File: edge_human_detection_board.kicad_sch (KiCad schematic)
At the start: 1 part

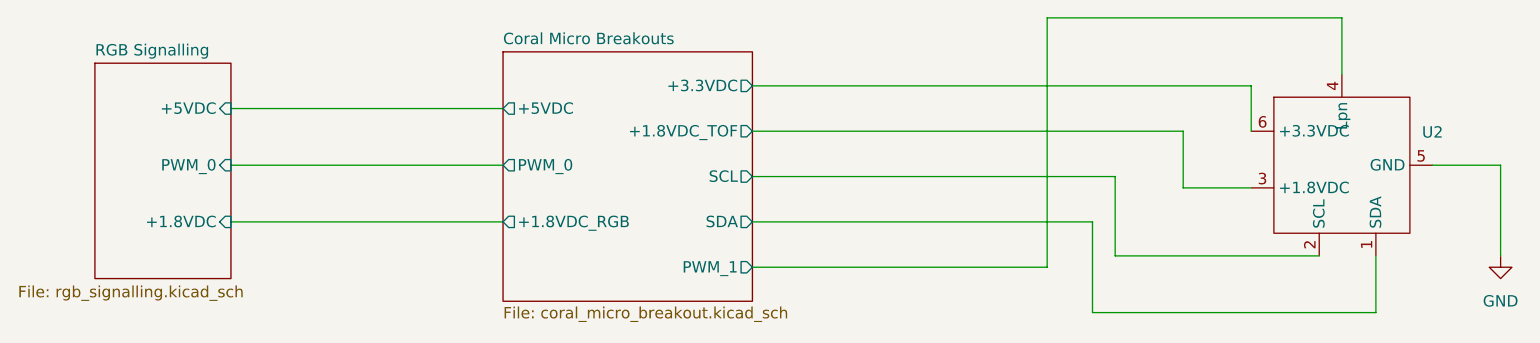
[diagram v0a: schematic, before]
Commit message: latest updates, up to v2
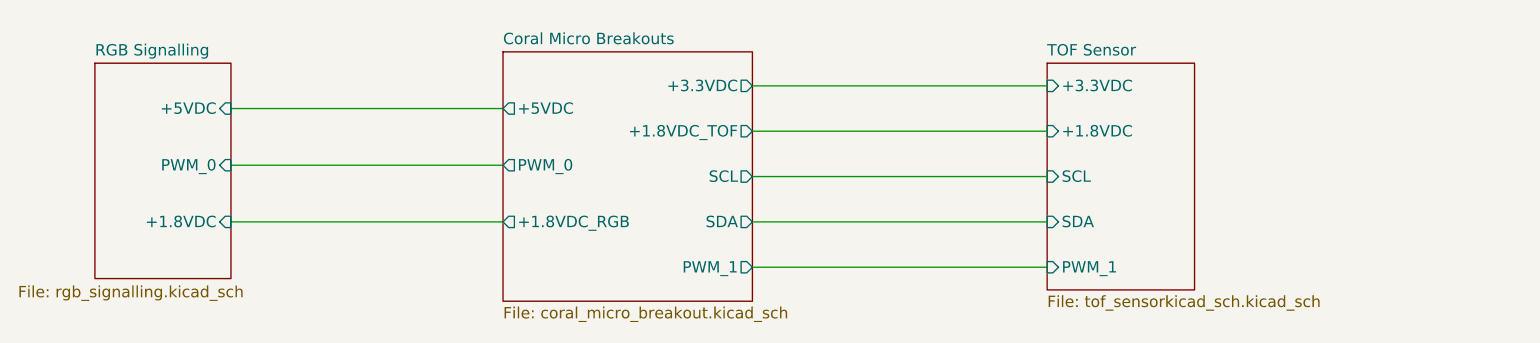
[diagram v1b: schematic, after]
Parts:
- removed U2: ~, 00_parts_lib:TOF_MODULE, symbol 00_project_parts:tof_module
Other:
- added sheet TOF Sensor (tof_sensorkicad_sch.kicad_sch)
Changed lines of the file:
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@@
-	(wire
-		(pts
-			(xy 203.2 73.66) (xy 203.2 68.58)
-		)
-		(stroke
-			(width 0)
-			(type default)
-		)
-	)
-	(wire
-		(pts
-			(xy 223.52 77.47) (xy 231.14 77.47)
-		)
-		(stroke
-			(width 0)
-			(type default)
-		)
-	)
-	(wire
-		(pts
-			(xy 195.58 73.66) (xy 195.58 80.01)
-		)
-		(stroke
-			(width 0)
-			(type default)
-		)
-	)
-	(wire
-		(pts
-			(xy 180.34 60.96) (xy 213.36 60.96)
-		)
-		(stroke
-			(width 0)
-			(type default)
-		)
-	)
 	(wire
 		(pts
@@
 	(wire
 		(pts
-			(xy 231.14 77.47) (xy 231.14 87.63)
-		)
-		(stroke
-			(width 0)
-			(type default)
-		)
-	)
-	(wire
-		(pts
 			(xy 88.9 83.82) (xy 119.38 83.82)
 		)
@@
 	(wire
 		(pts
-			(xy 147.32 68.58) (xy 203.2 68.58)
-		)
-		(stroke
-			(width 0)
-			(type default)
-		)
-	)
-	(wire
-		(pts
-			(xy 147.32 78.74) (xy 187.96 78.74)
-		)
-		(stroke
-			(width 0)
-			(type default)
-		)
-	)
-	(wire
-		(pts
-			(xy 187.96 78.74) (xy 187.96 87.63)
-		)
-		(stroke
-			(width 0)
-			(type default)
-		)
-	)
-	(wire
-		(pts
-			(xy 195.58 80.01) (xy 203.2 80.01)
-		)
-		(stroke
-			(width 0)
-			(type default)
-		)
-	)
-	(wire
-		(pts
-			(xy 147.32 73.66) (xy 195.58 73.66)
+			(xy 147.32 68.58) (xy 180.34 68.58)
+		)
+		(stroke
+			(width 0)
+			(type default)
+		)
+	)
+	(wire
+		(pts
+			(xy 147.32 78.74) (xy 180.34 78.74)
+		)
+		(stroke
+			(width 0)
+			(type default)
+		)
+	)
+	(wire
+		(pts
+			(xy 147.32 73.66) (xy 180.34 73.66)
 		)
 		(stroke
@@
 	(wire
 		(pts
-			(xy 187.96 87.63) (xy 210.82 87.63)
-		)
-		(stroke
-			(width 0)
-			(type default)
-		)
-	)
-	(wire
-		(pts
-			(xy 217.17 93.98) (xy 217.17 87.63)
-		)
-		(stroke
-			(width 0)
-			(type default)
-		)
-	)
-	(wire
-		(pts
-			(xy 213.36 60.96) (xy 213.36 67.31)
-		)
-		(stroke
-			(width 0)
-			(type default)
-		)
-	)
-	(wire
-		(pts
-			(xy 185.42 83.82) (xy 185.42 93.98)
-		)
-		(stroke
-			(width 0)
-			(type default)
-		)
-	)
-	(wire
-		(pts
-			(xy 185.42 93.98) (xy 217.17 93.98)
-		)
-		(stroke
-			(width 0)
-			(type default)
-		)
-	)
-	(wire
-		(pts
-			(xy 180.34 88.9) (xy 180.34 60.96)
-		)
-		(stroke
-			(width 0)
-			(type default)
-		)
-	)
-	(wire
-		(pts
-			(xy 147.32 83.82) (xy 185.42 83.82)
-		)
-		(stroke
-			(width 0)
-			(type default)
-		)
-	)
-	(symbol
-		(lib_id "00_project_parts:tof_module")
-		(at 213.36 77.47 0)
-		(unit 1)
-		(exclude_from_sim no)
-		(in_bom yes)
-		(on_board yes)
-		(dnp no)
-		(fields_autoplaced yes)
-		(property "Reference" "U2"
-			(at 223.52 73.7868 0)
-			(effects
-				(font
-					(size 1.27 1.27)
-				)
-			)
-		)
-		(property "Value" "~"
-			(at 223.52 75.6919 0)
-			(effects
-				(font
-					(size 1.27 1.27)
-				)
-			)
-		)
-		(property "Footprint" "00_parts_lib:TOF_MODULE"
-			(at 213.36 77.47 0)
-			(effects
-				(font
-					(size 1.27 1.27)
-				)
-				(hide yes)
-			)
-		)
-		(property "Datasheet" ""
-			(at 213.36 77.47 0)
-			(effects
-				(font
-					(size 1.27 1.27)
-				)
-				(hide yes)
-			)
-		)
-		(property "Description" ""
-			(at 213.36 77.47 0)
-			(effects
-				(font
-					(size 1.27 1.27)
-				)
-				(hide yes)
-			)
-		)
-		(pin "4"
-		)
-		(pin "1"
-		)
-		(pin "2"
-		)
-		(pin "5"
-		)
-		(pin "3"
-		)
-		(pin "6"
-		)
-		(instances
-			(project ""
-				(path "/f7edb1cc-a42a-4cc0-9a6f-d9bd2b944353"
-					(reference "U2")
-					(unit 1)
-				)
-			)
-		)
-	)
-	(symbol
-		(lib_id "power:GND")
-		(at 231.14 87.63 0)
-		(unit 1)
-		(exclude_from_sim no)
-		(in_bom yes)
-		(on_board yes)
-		(dnp no)
-		(fields_autoplaced yes)
-		(property "Reference" "#PWR017"
-			(at 231.14 93.98 0)
-			(effects
-				(font
-					(size 1.27 1.27)
-				)
-				(hide yes)
-			)
-		)
-		(property "Value" "GND"
-			(at 231.14 92.71 0)
-			(effects
-				(font
-					(size 1.27 1.27)
-				)
-			)
-		)
-		(property "Footprint" ""
-			(at 231.14 87.63 0)
-			(effects
-				(font
-					(size 1.27 1.27)
-				)
-				(hide yes)
-			)
-		)
-		(property "Datasheet" ""
-			(at 231.14 87.63 0)
-			(effects
-				(font
-					(size 1.27 1.27)
-				)
-				(hide yes)
-			)
-		)
-		(property "Description" "Power symbol creates a global label with name \"GND\" , ground"
-			(at 231.14 87.63 0)
-			(effects
-				(font
-					(size 1.27 1.27)
-				)
-				(hide yes)
-			)
-		)
-		(pin "1"
-		)
-		(instances
-			(project ""
-				(path "/f7edb1cc-a42a-4cc0-9a6f-d9bd2b944353"
-					(reference "#PWR017")
-					(unit 1)
-				)
-			)
+			(xy 147.32 83.82) (xy 180.34 83.82)
+		)
+		(stroke
+			(width 0)
+			(type default)
 		)
 	)
@@
 				)
 			)
+		)
+	)
+	(sheet
+		(at 180.34 66.04)
+		(size 16.51 25.4)
+		(fields_autoplaced yes)
+		(stroke
+			(width 0.1524)
+			(type solid)
+		)
+		(fill
+			(color 0 0 0 0.0000)
+		)
+		(property "Sheetname" "TOF Sensor"
+			(at 180.34 65.3284 0)
+			(effects
+				(font
+					(size 1.27 1.27)
+				)
+				(justify left bottom)
+			)
+		)
+		(property "Sheetfile" "tof_sensorkicad_sch.kicad_sch"
+			(at 180.34 92.0246 0)
+			(effects
+				(font
+					(size 1.27 1.27)
+				)
+				(justify left top)
+			)
+		)
+		(pin "PWM_1" input
+			(at 180.34 88.9 180)
+			(effects
+				(font
+					(size 1.27 1.27)
+				)
+				(justify left)
+			)
+		)
+		(pin "+1.8VDC" input
+			(at 180.34 73.66 180)
+			(effects
+				(font
+					(size 1.27 1.27)
+				)
+				(justify left)
+			)
+		)
+		(pin "SDA" input
+			(at 180.34 83.82 180)
+			(effects
+				(font
+					(size 1.27 1.27)
+				)
+				(justify left)
+			)
+		)
+		(pin "+3.3VDC" input
+			(at 180.34 68.58 180)
+			(effects
+				(font
+					(size 1.27 1.27)
+				)
+				(justify left)
+			)
+		)
+		(pin "SCL" input
+			(at 180.34 78.74 180)
+			(effects
+				(font
+					(size 1.27 1.27)
+				)
+				(justify left)
+			)
+		)
+		(instances
+			(project "edge_human_detection_board"
+				(path "/f7edb1cc-a42a-4cc0-9a6f-d9bd2b944353"
+					(page "4")
+				)
+			)
